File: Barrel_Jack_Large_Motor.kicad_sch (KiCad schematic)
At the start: 9 parts, among them J15 Barrel_Jack, J16 Barrel_Jack, J17 Barrel_Jack, J18 Barrel_Jack, J19 Barrel_Jack, J20 Barrel_Jack, U27 L298N, U28 L298N, U29 L298N

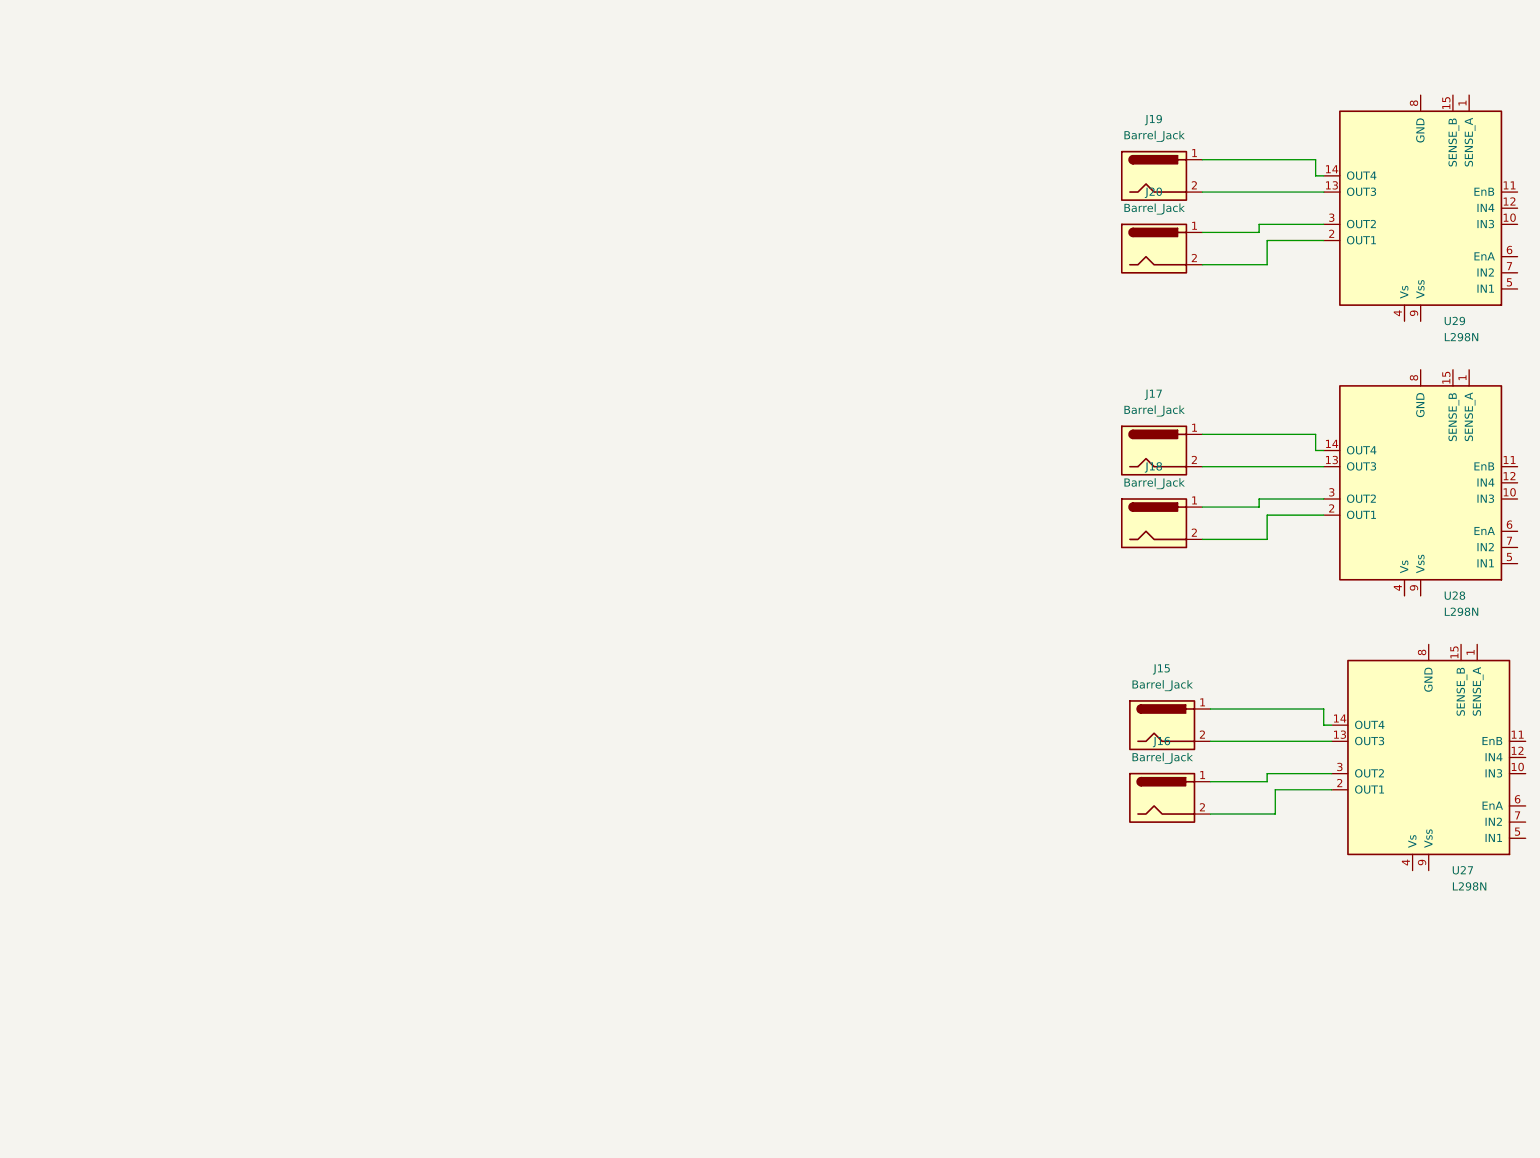
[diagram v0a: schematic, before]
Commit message: motor layout
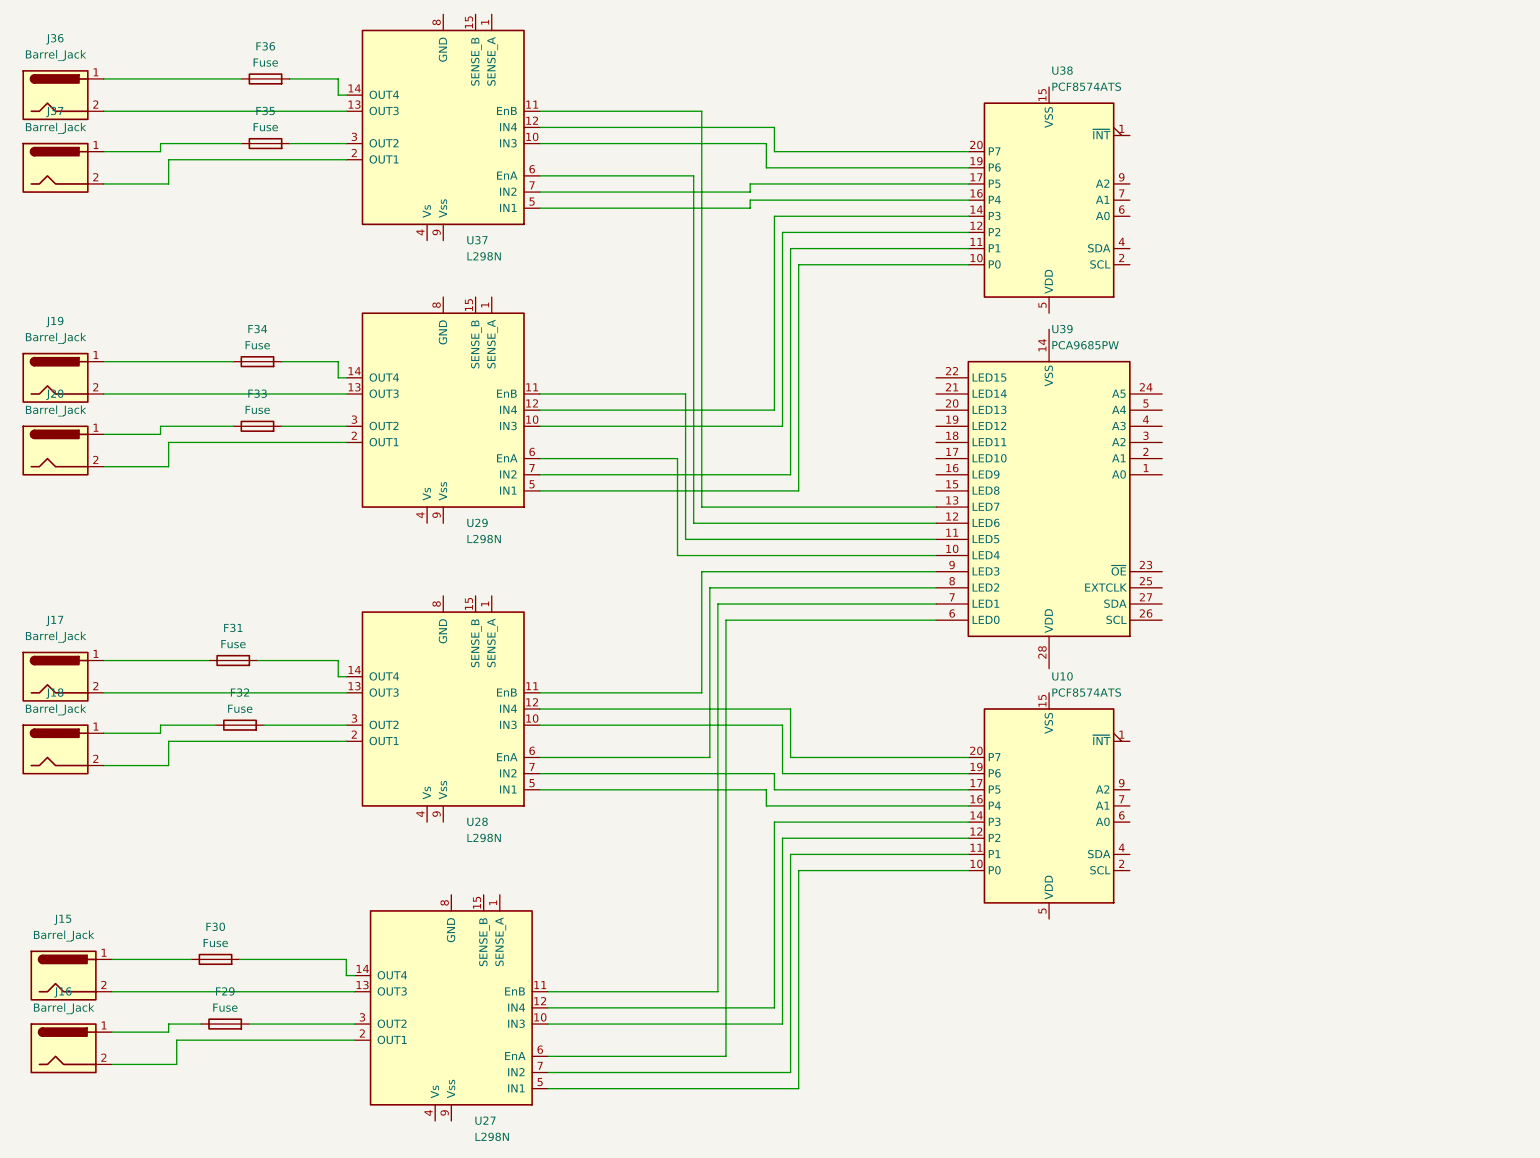
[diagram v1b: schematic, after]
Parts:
- added F29, F30, F31, F32, F33, F34, F35, F36: Fuse, symbol Device:Fuse
- added J36, J37: Barrel_Jack, symbol Connector:Barrel_Jack
- added U10, U38: PCF8574ATS, Package_SO:SSOP-20_4.4x6.5mm_P0.65mm, symbol Interface_Expansion:PCF8574ATS
- added U37: L298N, Package_TO_SOT_THT:TO-220-15_P2.54x2.54mm_StaggerOdd_Lead4.58mm_Vertical, symbol Driver_Motor:L298N
- added U39: PCA9685PW, Package_SO:TSSOP-28_4.4x9.7mm_P0.65mm, symbol Driver_LED:PCA9685PW
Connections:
- net at J15.1: now also F30.1; no longer U27.14 (OUT4)
- net at J17.1: now also F31.1; no longer U28.14 (OUT4)
- net at U28.10 (IN3): now also U10.19 (P6)
- net at U28.11 (EnB): now also U39.9 (LED3)
- net at U28.12 (IN4): now also U10.20 (P7)
- net at U28.3 (OUT2): now also F32.2; no longer J18.1
- net at U28.5 (IN1): now also U10.16 (P4)
- net at U28.6 (EnA): now also U39.8 (LED2)
- net at U28.7 (IN2): now also U10.17 (P5)
- net at J19.1: now also F34.1; no longer U29.14 (OUT4)
- net at U29.10 (IN3): now also U38.12 (P2)
- net at U29.11 (EnB): now also U39.11 (LED5)
- net at U29.12 (IN4): now also U38.14 (P3)
- net at J20.1: now also F33.1; no longer U29.3 (OUT2)
- net at U29.5 (IN1): now also U38.10 (P0)
- net at U29.6 (EnA): now also U39.10 (LED4)
- net at U29.7 (IN2): now also U38.11 (P1)
- net at J16.1: now also F29.1; no longer U27.3 (OUT2)
- net at U27.10 (IN3): now also U10.12 (P2)
- net at U27.11 (EnB): now also U39.7 (LED1)
- net at U27.12 (IN4): now also U10.14 (P3)
- net at U27.5 (IN1): now also U10.10 (P0)
- net at U27.6 (EnA): now also U39.6 (LED0)
- net at U27.7 (IN2): now also U10.11 (P1)
- new net: F36.1, J36.1
- new net: J36.2, U37.13 (OUT3)
- new net: F36.2, U37.14 (OUT4)
- new net: U37.10 (IN3), U38.19 (P6)
- new net: U37.11 (EnB), U39.13 (LED7)
- new net: U37.12 (IN4), U38.20 (P7)
- new net: J37.2, U37.2 (OUT1)
- new net: F35.2, U37.3 (OUT2)
- new net: U37.5 (IN1), U38.16 (P4)
- new net: U37.6 (EnA), U39.12 (LED6)
- new net: U37.7 (IN2), U38.17 (P5)
- new net: F29.2, U27.3 (OUT2)
- new net: F31.2, U28.14 (OUT4)
- new net: F33.2, U29.3 (OUT2)
- new net: F32.1, J18.1
- new net: F30.2, U27.14 (OUT4)
- new net: F34.2, U29.14 (OUT4)
- new net: F35.1, J37.1
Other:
- moved on the sheet: J15, J16, J17, J18, J19, J20, U27, U28, U29
